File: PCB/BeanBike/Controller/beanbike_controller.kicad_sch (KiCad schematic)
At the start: 1 part, among them U1 ESP32-WROOM-32

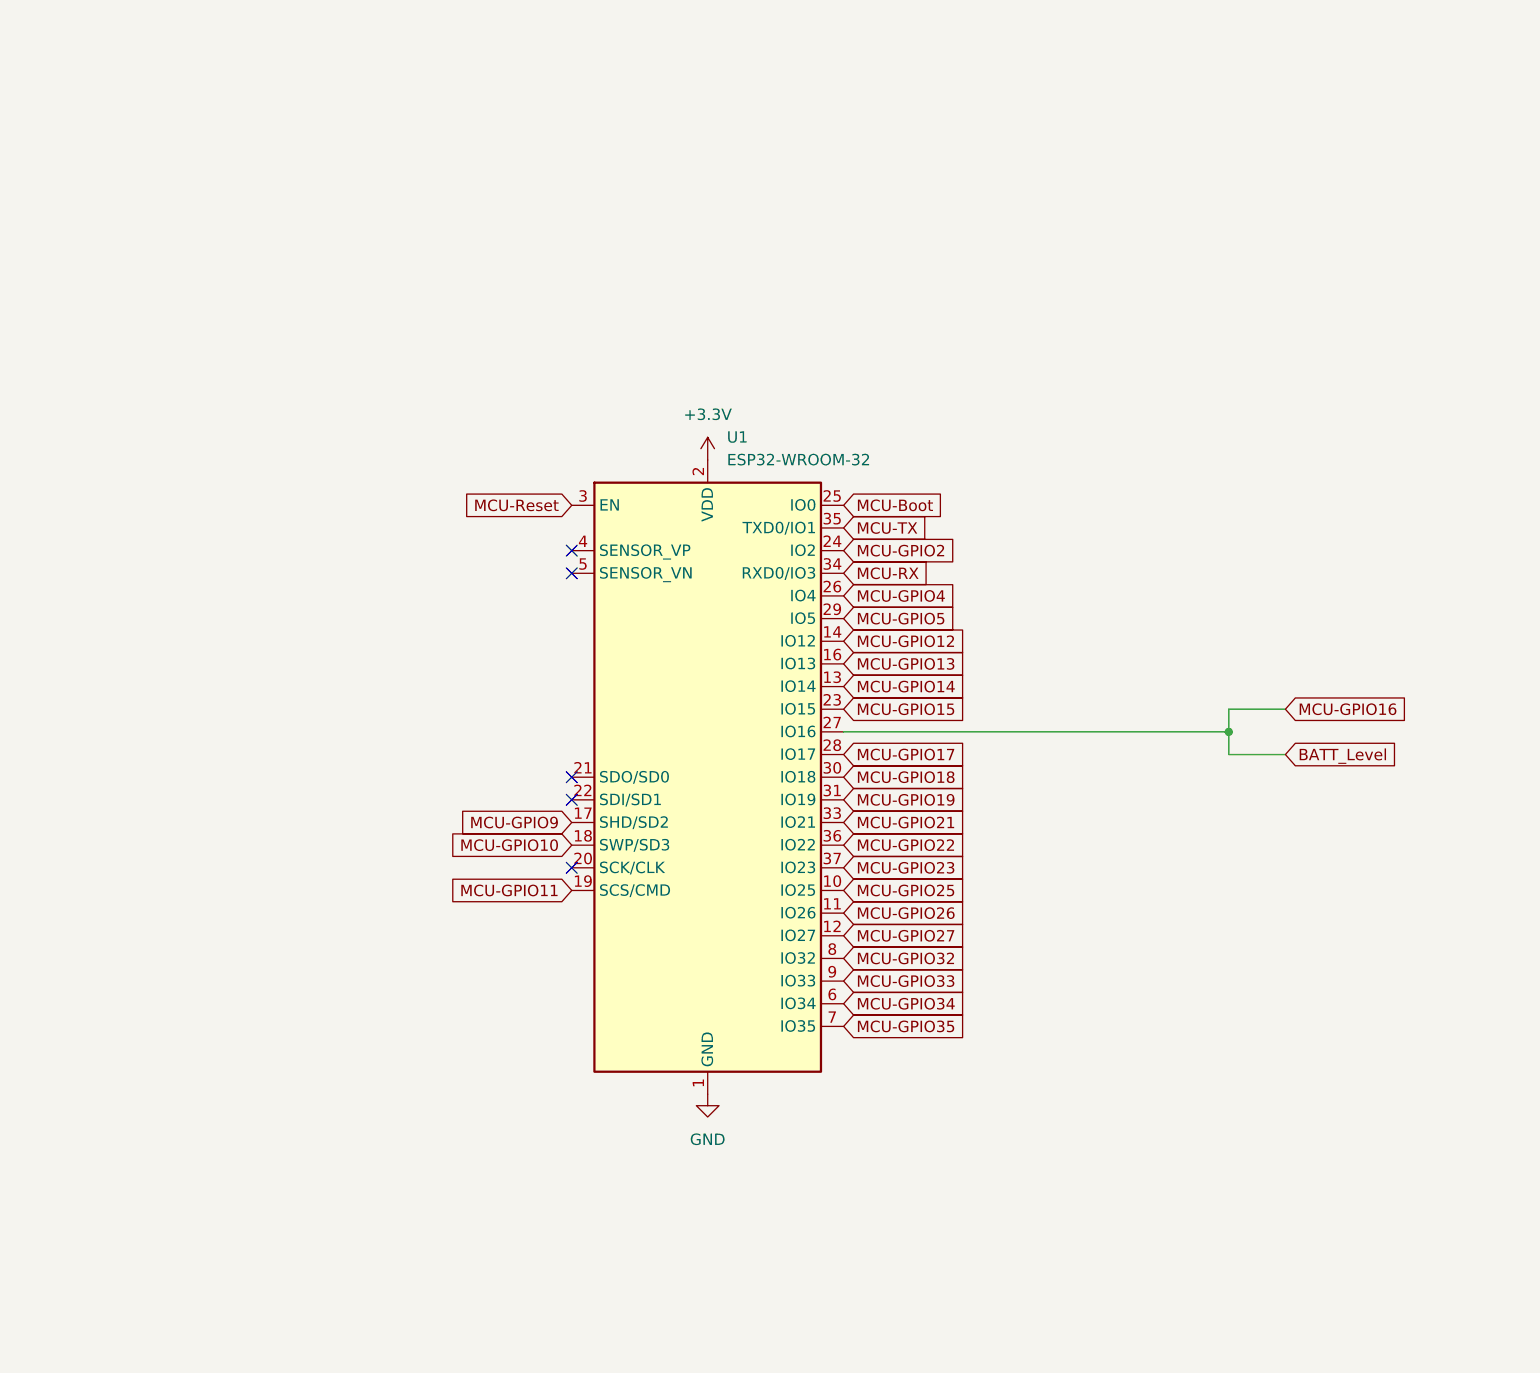
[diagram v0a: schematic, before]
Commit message: Forgot to commit
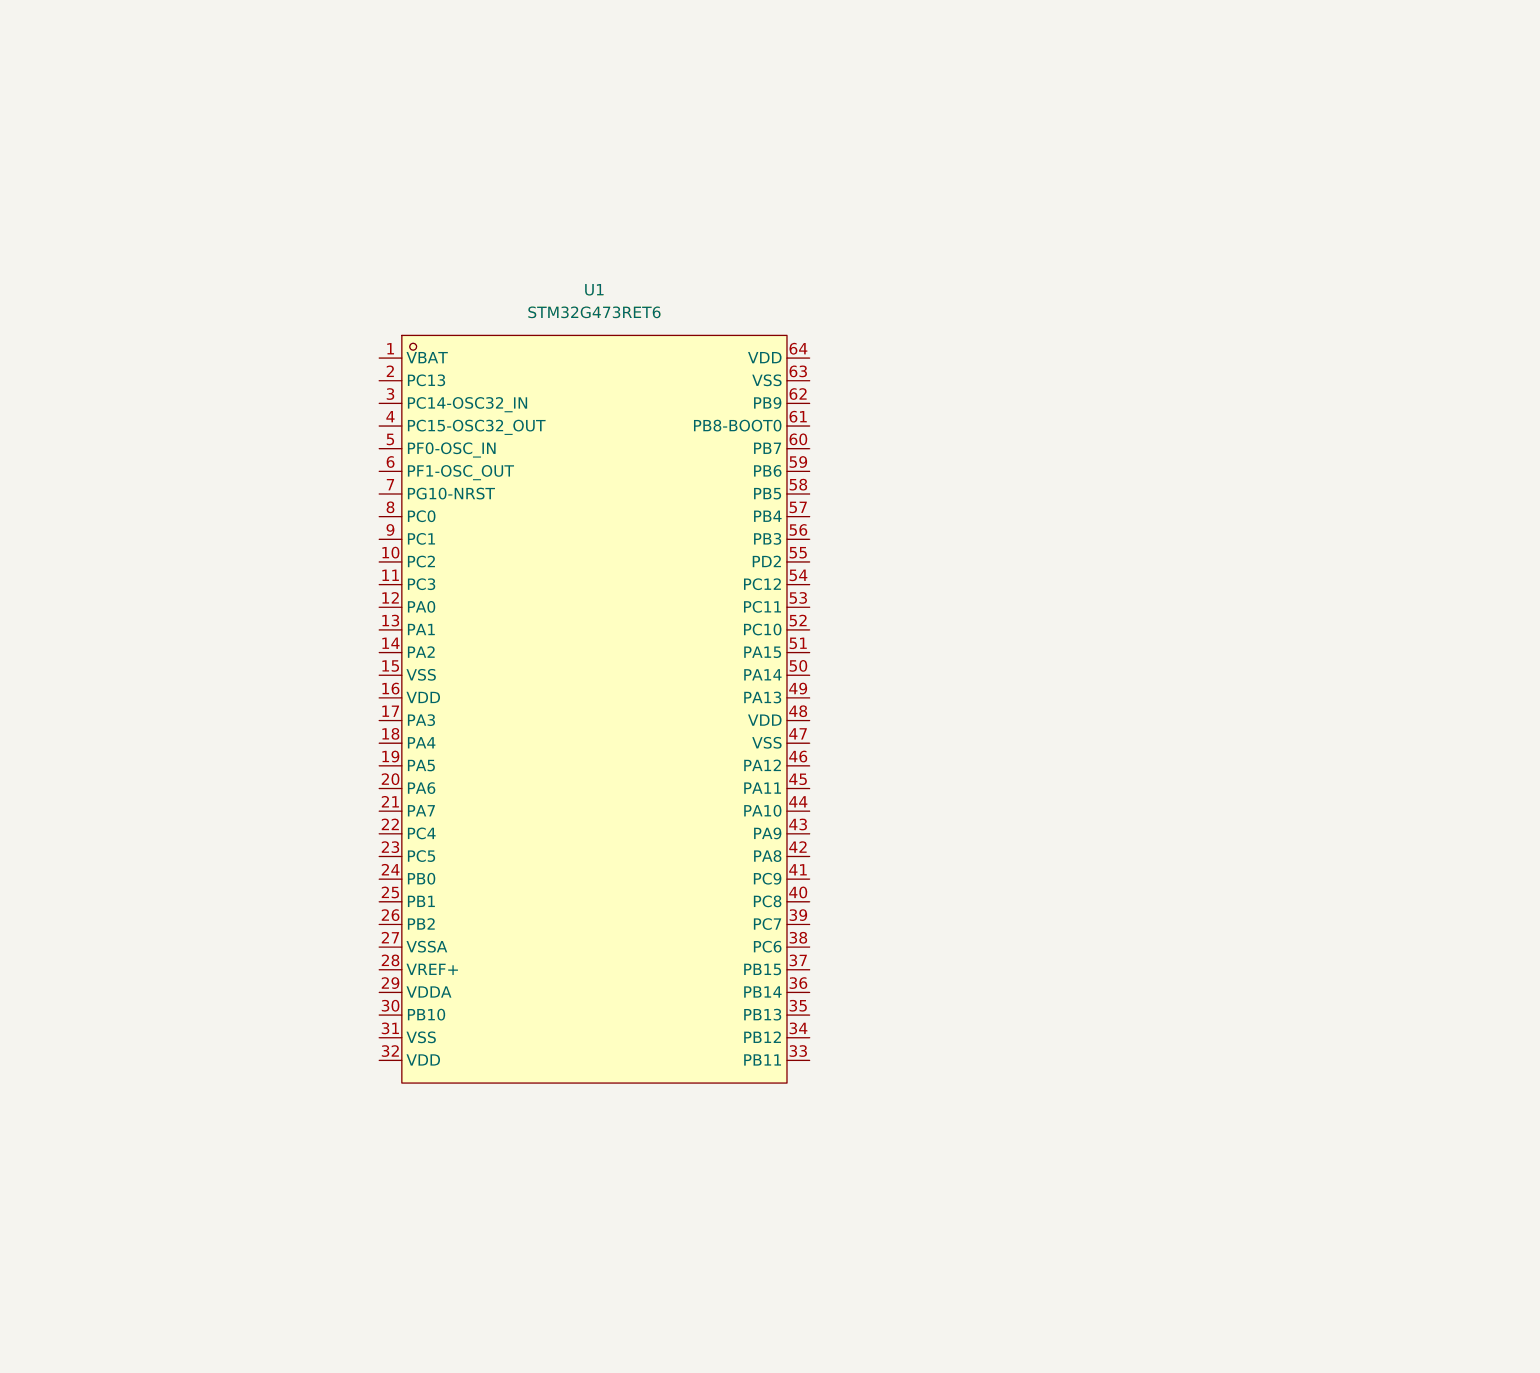
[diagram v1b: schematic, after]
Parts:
- removed U1: ESP32-WROOM-32, RF_Module:ESP32-WROOM-32, symbol RF_Module:ESP32-WROOM-32
- added U1: STM32G473RET6, easyeda2kicad:LQFP-64_L10.0-W10.0-P0.50-LS12.0-BL, symbol easyeda2kicad:STM32G473RET6
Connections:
- no-connect marks 5 -> 0

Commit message: STM32
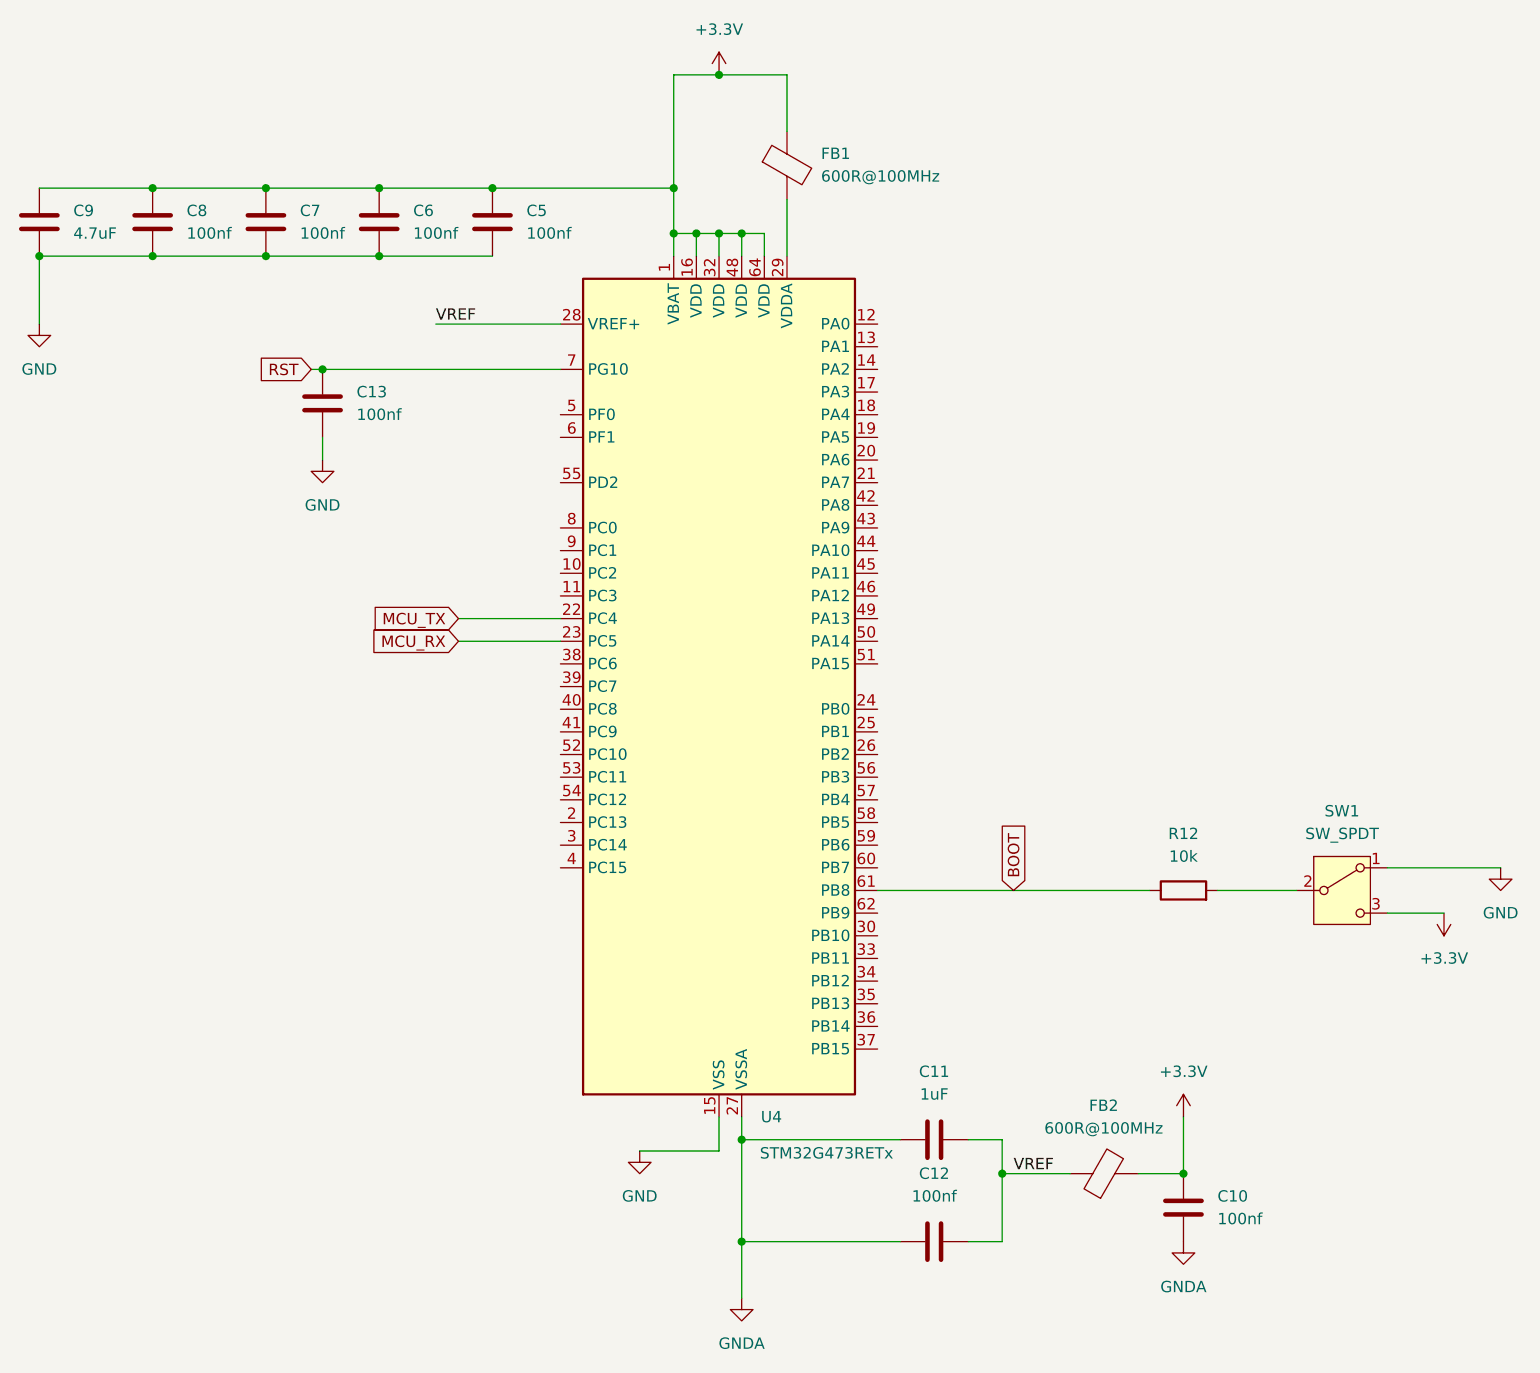
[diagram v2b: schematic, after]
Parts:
- removed U1: STM32G473RET6, easyeda2kicad:LQFP-64_L10.0-W10.0-P0.50-LS12.0-BL, symbol easyeda2kicad:STM32G473RET6
- added C10, C12, C13, C5, C6, C7, C8: 100nf, symbol Device:C
- added C11: 1uF, symbol Device:C
- added C9: 4.7uF, symbol Device:C
- added FB1, FB2: 600R@100MHz, symbol Device:FerriteBead
- added R12: 10k, symbol Device:R
- added SW1: SW_SPDT, symbol Switch:SW_SPDT
- added U4: STM32G473RETx, Package_QFP:LQFP-64_10x10mm_P0.5mm, symbol MCU_ST_STM32G4:STM32G473RETx
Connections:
- new net: R12.2, SW1.2 (B)
- new net: FB1.2, U4.29 (VDDA)
- new net +3.3V: C10.1, C5.1, C6.1, C7.1, C8.1, C9.1, FB1.1, FB2.2, SW1.3 (C), U4.1 (VBAT), U4.16 (VDD), U4.32 (VDD), U4.48 (VDD), U4.64 (VDD)
- new net BOOT: R12.1, U4.61 (PB8)
- new net GND: C13.2, C5.2, C6.2, C7.2, C8.2, C9.2, SW1.1 (A), U4.15 (VSS), U4.31 (VSS), U4.47 (VSS), U4.63 (VSS)
- new net GNDA: C10.2, C11.1, C12.1, U4.27 (VSSA)
- new net MCU_RX: U4.23 (PC5)
- new net MCU_TX: U4.22 (PC4)
- new net RST: C13.1, U4.7 (PG10)
- new net VREF: C11.2, C12.2, FB2.1, U4.28 (VREF+)
